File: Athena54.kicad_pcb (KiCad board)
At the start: 4 copper layers, 137.4 x 108 mm, 106 parts, among them J1 BATT, J2 HRO_TYPE-C-31-M-12, J3 JTAG_TC2030, J4 RGB, Q1 2N7002, Q2 2N7002, Q3 AO3407, SW1 POWER, SW10 MX Hotswap, SW11 MX Hotswap, SW12 MX Hotswap, SW13 MX Hotswap, SW14 MX Hotswap, SW15 MX Hotswap, SW16 MX Hotswap, SW17 MX Hotswap, SW18 MX Hotswap, SW19 MX Hotswap, SW2 MX Hotswap, SW20 MX Hotswap, SW21 MX Hotswap, SW22 MX Hotswap, SW23 MX Hotswap, SW24 MX Hotswap, SW25 MX Hotswap, SW26 MX Hotswap, SW27 MX Hotswap, SW28 MX Hotswap, SW29 RESET, SW3 MX Hotswap, SW4 MX Hotswap, SW5 MX Hotswap, SW6 MX Hotswap, SW7 MX Hotswap, SW8 MX Hotswap, SW9 MX Hotswap, U1 BQ24075RGT, U2 MAX17048, U3 USBLC6-2SC6, U4 nRF52840_moko_mk08

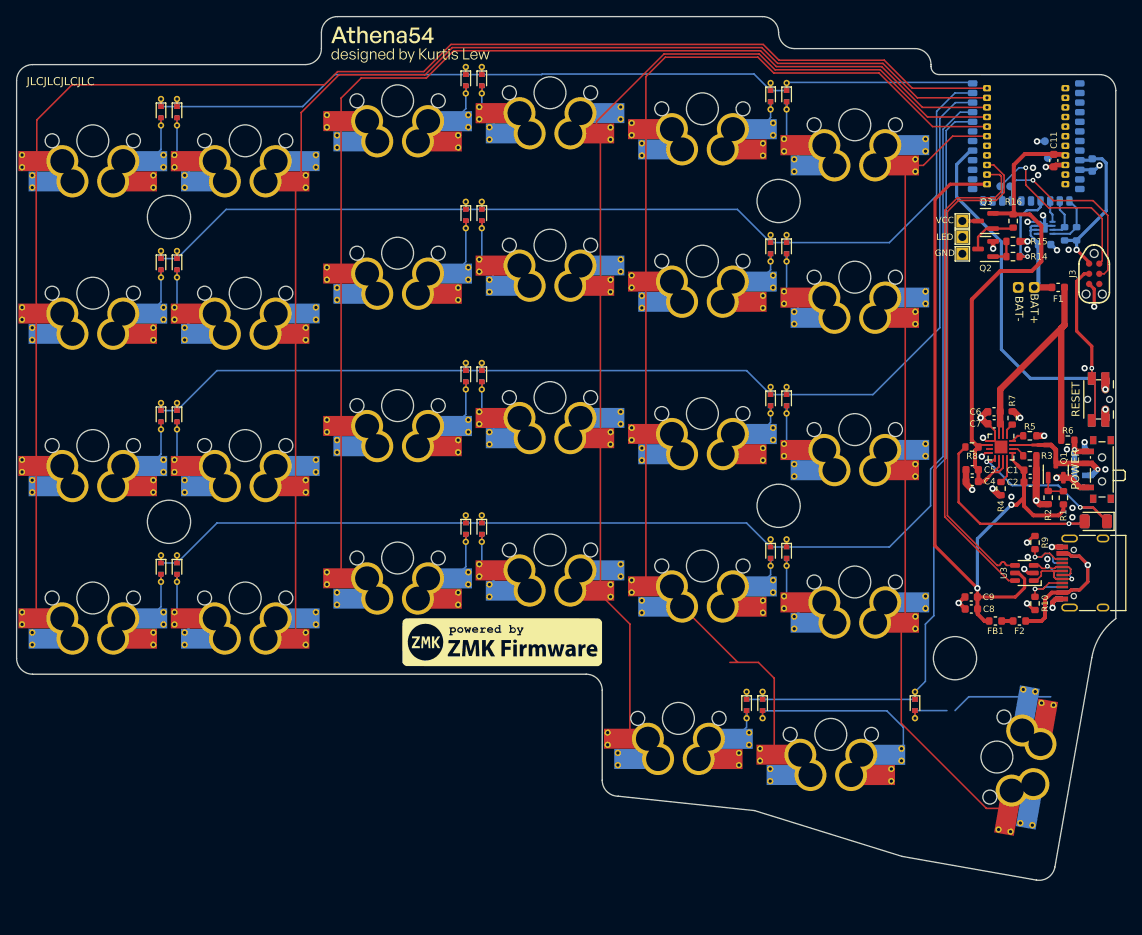
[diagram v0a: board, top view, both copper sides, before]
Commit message: feat(pcb): Version 0.2
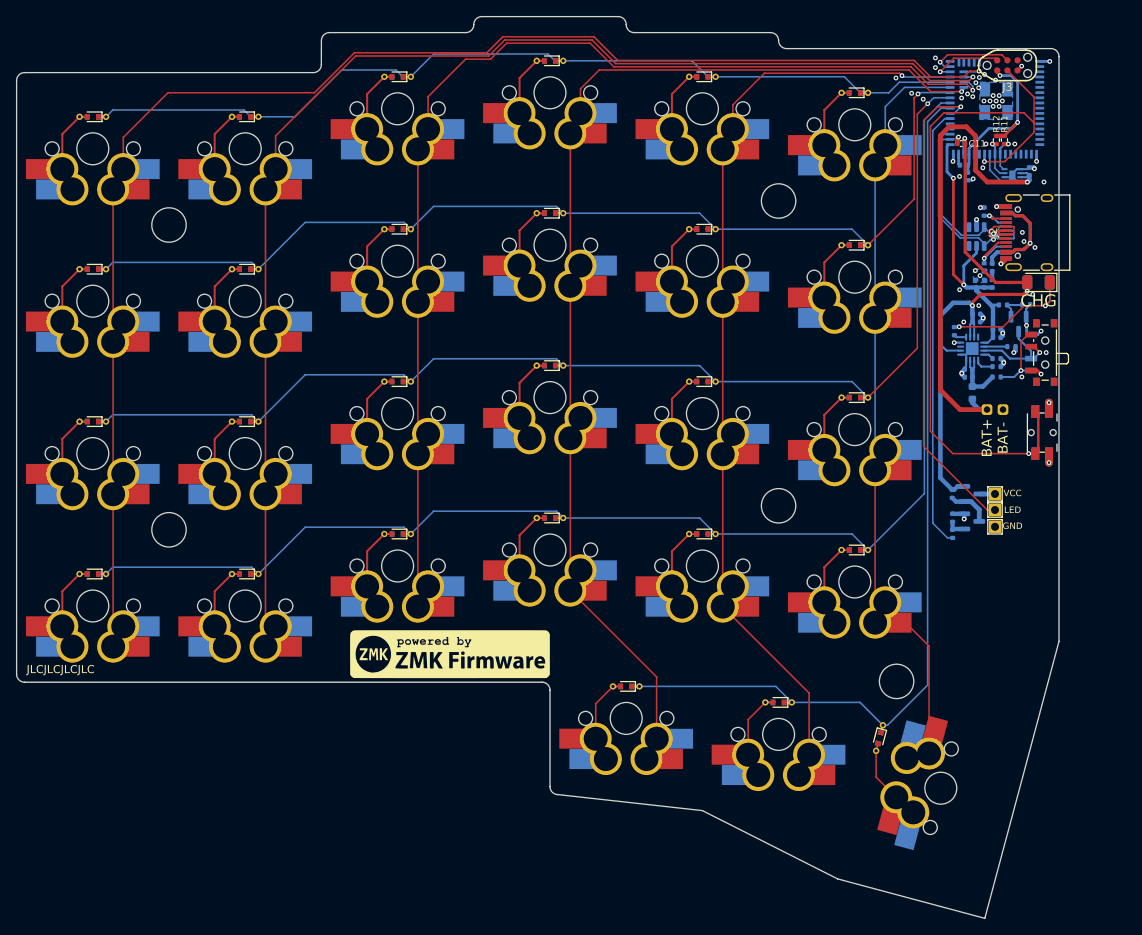
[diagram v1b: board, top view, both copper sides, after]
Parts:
- removed C12: 100nF, Capacitor_SMD:C_0603_1608Metric
- removed G*** (x2): LOGO, Conejo:Athena54
- removed R15, R16: 10K, Resistor_SMD:R_0603_1608Metric
- removed the R8 at (109.9, 39.3)
- added C10: 4.7uF, Capacitor_SMD:C_0402_1005Metric, B.Cu at (109.4, 5.45)
- added L1: NC, Inductor_SMD:L_0402_1005Metric, B.Cu at (108.9, 4.05)
- added R10: 100R, Resistor_SMD:R_0402_1005Metric, B.Cu at (107.5, 50.1)
- added R11: 1K5, Resistor_SMD:R_0402_1005Metric, F.Cu at (114.0, 0.90)
- C1, C2, C4, C5, C6, C7, C8, C9: footprint Capacitor_SMD:C_0603_1608Metric -> Capacitor_SMD:C_0402_1005Metric; moved to B.Cu
- C11, C3: footprint Capacitor_SMD:C_0603_1608Metric -> Capacitor_SMD:C_0402_1005Metric
- F1, J1, J4, Q1, Q2, Q3, U1: moved to B.Cu
- F2: footprint Fuse:Fuse_0603_1608Metric -> Fuse:Fuse_0402_1005Metric; moved to B.Cu
- FB1: footprint Inductor_SMD:L_0603_1608Metric -> Inductor_SMD:L_0402_1005Metric; moved to B.Cu
- G1: moved to F.Cu
- G2: renamed from G1; moved to B.Cu
- H1, H2, H3, H4, H5: footprint Athena54:MountingHole_5.4mm -> Athena54:MountingHole_4.3mm
- J2: footprint Conejo:USB_C_Receptacle_HRO_TYPE-C-31-M-12 (Reversible) -> Athena54:USB_C_Receptacle_HRO_TYPE-C-31-M-12 (Reversible)
- R1, R2, R3: footprint Resistor_SMD:R_0603_1608Metric -> Resistor_SMD:R_0402_1005Metric; moved to B.Cu
- R12: footprint Resistor_SMD:R_0603_1608Metric -> Resistor_SMD:R_0402_1005Metric; moved to F.Cu
- R13: value 1K5 -> 10K; footprint Resistor_SMD:R_0603_1608Metric -> Resistor_SMD:R_0402_1005Metric
- R14: value 100 -> 10K; footprint Resistor_SMD:R_0603_1608Metric -> Resistor_SMD:R_0402_1005Metric; moved to B.Cu
- R4: value RLIM -> RSET; footprint Resistor_SMD:R_0603_1608Metric -> Resistor_SMD:R_0402_1005Metric; moved to B.Cu
- R5: value RSET -> 100K; footprint Resistor_SMD:R_0603_1608Metric -> Resistor_SMD:R_0402_1005Metric; moved to B.Cu
- R6: value 100K -> 10K; footprint Resistor_SMD:R_0603_1608Metric -> Resistor_SMD:R_0402_1005Metric; moved to B.Cu
- R7: value 10K -> 1K5; footprint Resistor_SMD:R_0603_1608Metric -> Resistor_SMD:R_0402_1005Metric; moved to B.Cu
- R8: renamed from R9; footprint Resistor_SMD:R_0603_1608Metric -> Resistor_SMD:R_0402_1005Metric; moved to B.Cu
- R9: renamed from R10; footprint Resistor_SMD:R_0603_1608Metric -> Resistor_SMD:R_0402_1005Metric; moved to B.Cu
- SW10, SW11, SW12, SW13, SW18, SW19, SW2, SW20, SW21, SW22, SW23, SW3, SW4, SW5: footprint Athena54:MXOnly-1U-Hotswap-Antishear (reversible) -> Athena54:MXOnly-1U-Hotswap (Reversible); moved to F.Cu
- SW14, SW15, SW16, SW17, SW24, SW25, SW26, SW27, SW6, SW7, SW8, SW9: footprint Athena54:MXOnly-1U-Hotswap-Antishear (reversible) -> Athena54:MXOnly-1U-Hotswap (Reversible)
- SW28: footprint Athena54:MXOnly-1.5U-Hotswap-Antishear (reversible) -> Athena54:MXOnly-1.5U-Hotswap (Reversible)
- U3: value USBLC6-2SC6 -> SRV05-4; moved to B.Cu
- U4: value nRF52840_moko_mk08 -> MS88SF3; footprint marbastlib-various:nRF52840_moko_mk08 -> Athena54:MS88SF3
- moved F2 44.3 mm to (112.4, 16.8), turned to -90 degrees
- moved J2 43.1 mm to (118.2, 12.5)
- moved R9 42.5 mm to (111.4, 16.8)
- moved U3 42.5 mm to (110.5, 13.0), turned to -90 degrees
- moved FB1 42.2 mm to (112.4, 18.9), turned to -90 degrees
- moved R8 41.9 mm to (111.4, 9.85)
- moved C8 40.7 mm to (111.4, 18.9), turned to -90 degrees
- moved C9 39.2 mm to (110.4, 18.9), turned to -90 degrees
- moved R13 38.2 mm to (107.5, 48.1)
- moved J4 34.4 mm to (112.8, 47.1), turned to 180 degrees
- moved Q3 34.2 mm to (109.9, 45.1), turned to 0 degrees
- moved Q2 34.1 mm to (109.9, 48.6), turned to 0 degrees
- moved D1 30.7 mm to (118.2, 18.7)
- moved R14 30.6 mm to (107.4, 45.1), turned to 90 degrees
- moved J3 28.2 mm to (114.3, -8.43), turned to 0 degrees
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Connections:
- D1 pad 1: /Power Management/CHG -> Net-(D1-Pad1)
- D1 pad 2: Net-(D1-Pad2) -> VDDH
- J2 pad A6: DI+ -> D+
- J2 pad A7: DI- -> D-
- J2 pad B6: DI+ -> D+
- J2 pad B7: DI- -> D-
- J4 pad 2: LED -> LED_MOSI
- R12 pad 1: SDA -> SCL
- R13 pad 1: SCL -> GND
- R13 pad 2: VDD -> Net-(Q2-Pad1)
- R14 pad 1: EXT_PWR_EN -> Net-(Q2-Pad3)
- R14 pad 2: Net-(Q2-Pad1) -> VDDH
- R4 pad 2: /Power Management/ILIM -> /Power Management/ISET
- R5 pad 1: GND -> Net-(R5-Pad1)
- R5 pad 2: /Power Management/ISET -> VBAT
- R6 pad 1: Net-(R6-Pad1) -> GND
- R6 pad 2: VBAT -> /Power Management/TS
- R7 pad 1: GND -> /Power Management/CHG
- R7 pad 2: /Power Management/TS -> Net-(D1-Pad1)
- SW1 pad 3: Net-(R6-Pad1) -> Net-(R5-Pad1)
- U1 pad 12: /Power Management/ILIM -> unconnected-(U1-Pad12)
- U3 pad 1: DI- -> unconnected-(U3-Pad1)
- U3 pad 3: DI+ -> D-
- U3 pad 4: DO+ -> D+
- U3 pad 6: DO- -> unconnected-(U3-Pad6)
- U4 pad 1: unconnected-(U4-Pad1) -> GND
- U4 pad 10: GND -> unconnected-(U4-Pad10)
- U4 pad 13: SDA -> unconnected-(U4-Pad13)
- U4 pad 14: SCL -> unconnected-(U4-Pad14)
- U4 pad 15: ALERT -> unconnected-(U4-Pad15)
- U4 pad 16: EXT_PWR_EN -> unconnected-(U4-Pad16)
- U4 pad 18: unconnected-(U4-Pad18) -> GND
- U4 pad 19: SWDCLK -> unconnected-(U4-Pad19)
- U4 pad 20: SWDIO -> unconnected-(U4-Pad20)
- U4 pad 25: unconnected-(U4-Pad25) -> SDA
- U4 pad 26: unconnected-(U4-Pad26) -> SCL
- U4 pad 27: RESET -> ALERT
- U4 pad 28: unconnected-(U4-Pad28) -> RESET
- U4 pad 30: ROW5 -> unconnected-(U4-Pad30)
- U4 pad 31: ROW4 -> VDD
- U4 pad 32: ROW3 -> VDDH
- U4 pad 33: ROW2 -> DCCH
- U4 pad 34: ROW1 -> GND
- U4 pad 35: unconnected-(U4-Pad35) -> +5V
- U4 pad 36: unconnected-(U4-Pad36) -> D-
- U4 pad 37: unconnected-(U4-Pad37) -> D+
- U4 pad 39: GND -> unconnected-(U4-Pad39)
- U4 pad 40: unconnected-(U4-Pad40) -> EXT_PWR_EN
- U4 pad 41: unconnected-(U4-Pad41) -> LED_MOSI
- U4 pad 42: VDDH -> ROW5
- U4 pad 43: GND -> ROW4
- U4 pad 44: unconnected-(U4-Pad44) -> ROW3
- U4 pad 45: unconnected-(U4-Pad45) -> ROW2
- U4 pad 46: +5V -> COL6
- U4 pad 47: DO- -> ROW1
- U4 pad 48: DO+ -> COL5
- U4 pad 49: unconnected-(U4-Pad49) -> SWDIO
- U4 pad 50: unconnected-(U4-Pad50) -> SWDCLK
- U4 pad 51: COL6 -> unconnected-(U4-Pad51)
- U4 pad 52: COL5 -> unconnected-(U4-Pad52)
- U4 pad 53: COL4 -> unconnected-(U4-Pad53)
- U4 pad 54: COL3 -> unconnected-(U4-Pad54)
- U4 pad 55: COL2 -> unconnected-(U4-Pad55)
- U4 pad 56: COL1 -> unconnected-(U4-Pad56)
- U4 pad 57: GND -> COL1
- U4 pad 9: VDD -> unconnected-(U4-Pad9)
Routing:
- net DO+: track 62.4 -> 0.00 mm
- net DO-: track 62.2 -> 0.00 mm
- net +5V: track 101.7 -> 39.9 mm
- net LED_MOSI: track 0.00 -> 60.0 mm, vias 0 -> 1
- net +BATT: track 12.0 -> 61.4 mm, vias 0 -> 1
- net EXT_PWR_EN: track 10.3 -> 55.1 mm, vias 1 -> 0
- net D+: track 0.00 -> 30.8 mm, vias 0 -> 1
- net VBAT: track 37.8 -> 7.67 mm
- net RESET: track 65.7 -> 94.1 mm, vias 1 -> 2
- net D-: track 0.00 -> 27.3 mm, vias 0 -> 1
- net Net-(D1-Pad2): track 26.3 -> 0.00 mm, vias 1 -> 0
- net COL5: track 136.7 -> 112.2 mm, vias 0 -> 1
- net GND: track 64.2 -> 40.3 mm, vias 39 -> 60
- net /Power Management/CHG: track 23.4 -> 1.57 mm, vias 2 -> 0
- net Net-(D1-Pad1): track 0.00 -> 18.8 mm, vias 0 -> 2
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- added copper zone on B.Cu, net GND
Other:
- board size 137.4 x 108 mm -> 130.3 x 112.7 mm
- board text removed: "POWER"
- board text removed: "RESET"
